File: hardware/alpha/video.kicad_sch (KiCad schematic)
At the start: 84 parts, among them J2 VIDEO OUT, U4 AD768, U5 MAX4104, U6 TLE2082, U7 MAX4104

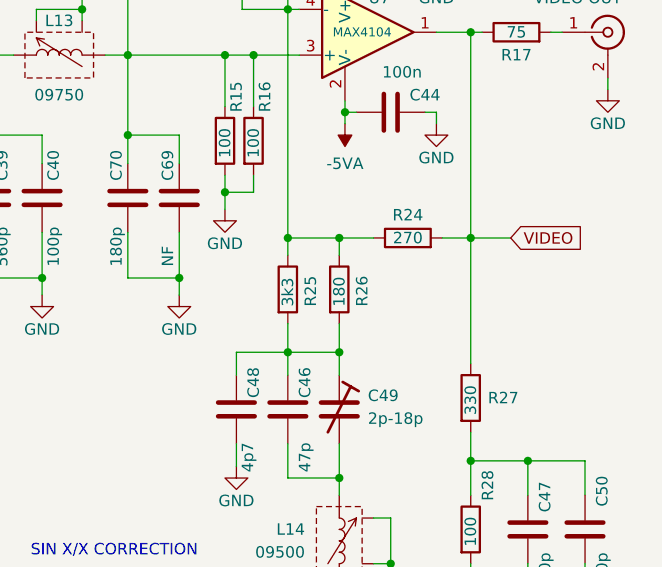
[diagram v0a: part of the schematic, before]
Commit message: WIP
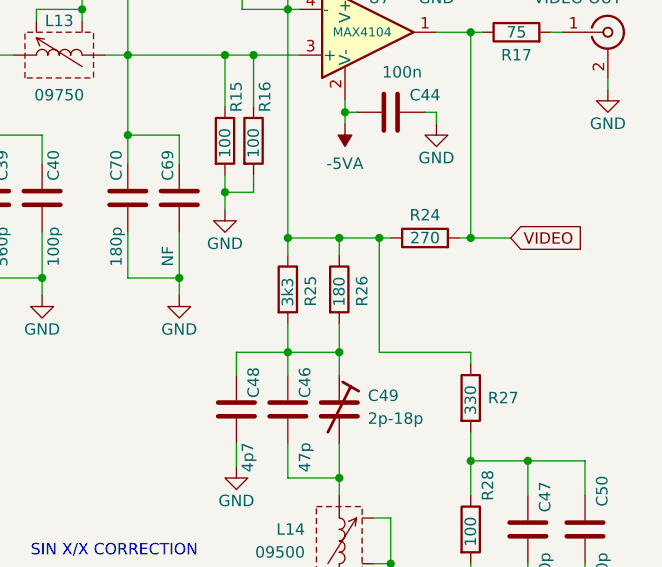
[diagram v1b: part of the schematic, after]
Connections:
- net VIDEO: no longer R27.1
- net at R19.2, R20.1, R24.1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: now also R27.1
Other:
- moved on the sheet: R24
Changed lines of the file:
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@@
   (junction (at 225.425 72.39) (diameter 0) (color 0 0 0 0)
   )
+  (junction (at 253.365 107.315) (diameter 0) (color 0 0 0 0)
+  )
   (junction (at 144.145 79.375) (diameter 0) (color 0 0 0 0)
   )
@@
     (stroke (width 0) (type default))
   )
-  (wire (pts (xy 252.73 107.315) (xy 248.92 107.315))
+  (wire (pts (xy 254.635 107.315) (xy 253.365 107.315))
     (stroke (width 0) (type default))
   )
@@
     (stroke (width 0) (type default))
   )
-  (wire (pts (xy 260.35 107.315) (xy 263.525 107.315))
+  (wire (pts (xy 262.255 107.315) (xy 263.525 107.315))
     (stroke (width 0) (type default))
   )
@@
     (stroke (width 0) (type default))
   )
+  (wire (pts (xy 253.365 107.315) (xy 248.92 107.315))
+    (stroke (width 0) (type default))
+  )
   (wire (pts (xy 93.98 132.08) (xy 93.98 134.62))
     (stroke (width 0) (type default))
@@
     (stroke (width 0) (type default))
   )
-  (wire (pts (xy 263.525 107.315) (xy 263.525 121.285))
-    (stroke (width 0) (type default))
-  )
   (wire (pts (xy 248.92 146.05) (xy 248.92 148.59))
     (stroke (width 0) (type default))
@@
     (stroke (width 0) (type default))
   )
+  (wire (pts (xy 263.525 120.015) (xy 253.365 120.015))
+    (stroke (width 0) (type default))
+  )
   (wire (pts (xy 252.73 138.43) (xy 254.635 138.43))
     (stroke (width 0) (type default))
@@
     (stroke (width 0) (type default))
   )
+  (wire (pts (xy 263.525 121.285) (xy 263.525 120.015))
+    (stroke (width 0) (type default))
+  )
   (wire (pts (xy 170.815 128.905) (xy 176.53 128.905))
     (stroke (width 0) (type default))
@@
     (stroke (width 0) (type default))
   )
+  (wire (pts (xy 253.365 120.015) (xy 253.365 107.315))
+    (stroke (width 0) (type default))
+  )
   (wire (pts (xy 175.895 59.69) (xy 179.705 59.69))
     (stroke (width 0) (type default))
@@
     )
   )
-  (symbol (lib_id "Device:R") (at 256.54 107.315 90) (unit 1)
+  (symbol (lib_id "Device:R") (at 258.445 107.315 90) (unit 1)
     (in_bom yes) (on_board yes) (dnp no)
-    (property "Reference" "R24" (at 256.54 104.775 90)
+    (property "Reference" "R24" (at 258.445 104.775 90)
       (effects (font (size 1.27 1.27)))
     )
-    (property "Value" "270" (at 256.54 107.315 90)
+    (property "Value" "270" (at 258.445 107.315 90)
       (effects (font (size 1.27 1.27)))
     )
-    (property "Footprint" "Resistor_SMD:R_0603_1608Metric" (at 256.54 109.093 90)
+    (property "Footprint" "Resistor_SMD:R_0603_1608Metric" (at 258.445 109.093 90)
       (effects (font (size 1.27 1.27)) hide)
     )
-    (property "Datasheet" "~" (at 256.54 107.315 0)
+    (property "Datasheet" "~" (at 258.445 107.315 0)
       (effects (font (size 1.27 1.27)) hide)
     )

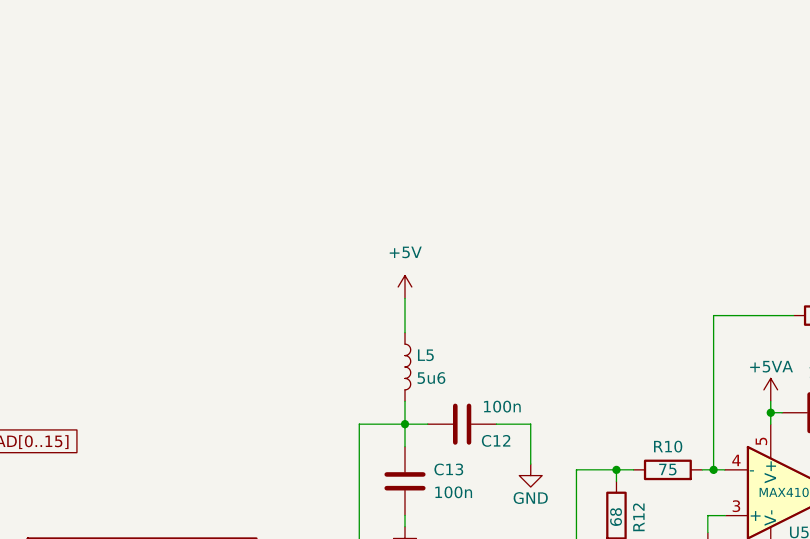
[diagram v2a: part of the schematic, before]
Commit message: WIP
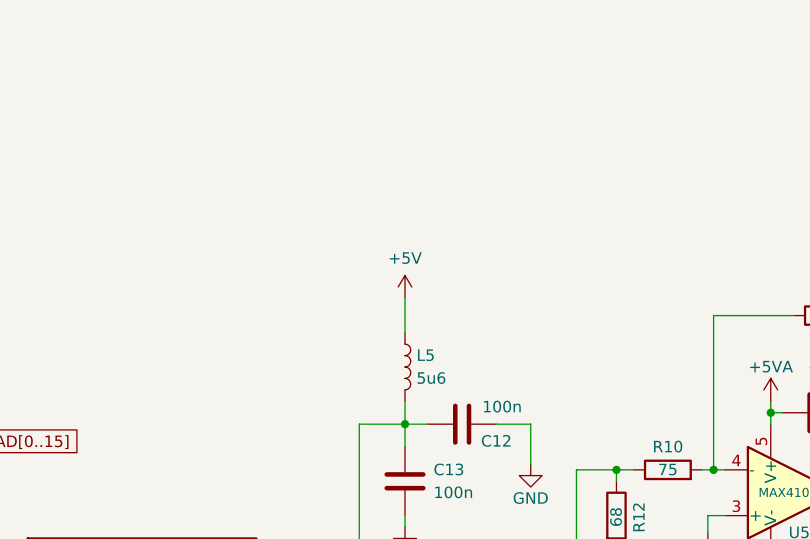
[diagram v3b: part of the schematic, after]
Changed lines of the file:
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@@
 	)
 	(symbol
-		(lib_name "KJL_ADJ:KJL_ADJ_SGL")
 		(lib_id "KJL_ADJ:KJL_ADJ_SGL")
 		(at 187.325 86.995 90)
@@
 		(on_board yes)
 		(dnp no)
-		(fields_autoplaced yes)
 		(property "Reference" "#PWR08"
 			(at 78.74 61.595 0)
@@
 		)
 		(property "Value" "+5V"
-			(at 78.74 52.705 0)
+			(at 78.74 53.34 0)
 			(effects
 				(font
